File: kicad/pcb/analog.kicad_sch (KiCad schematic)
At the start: 20 parts, among them U2 74HC4051, U5 OPA354AIDBVR

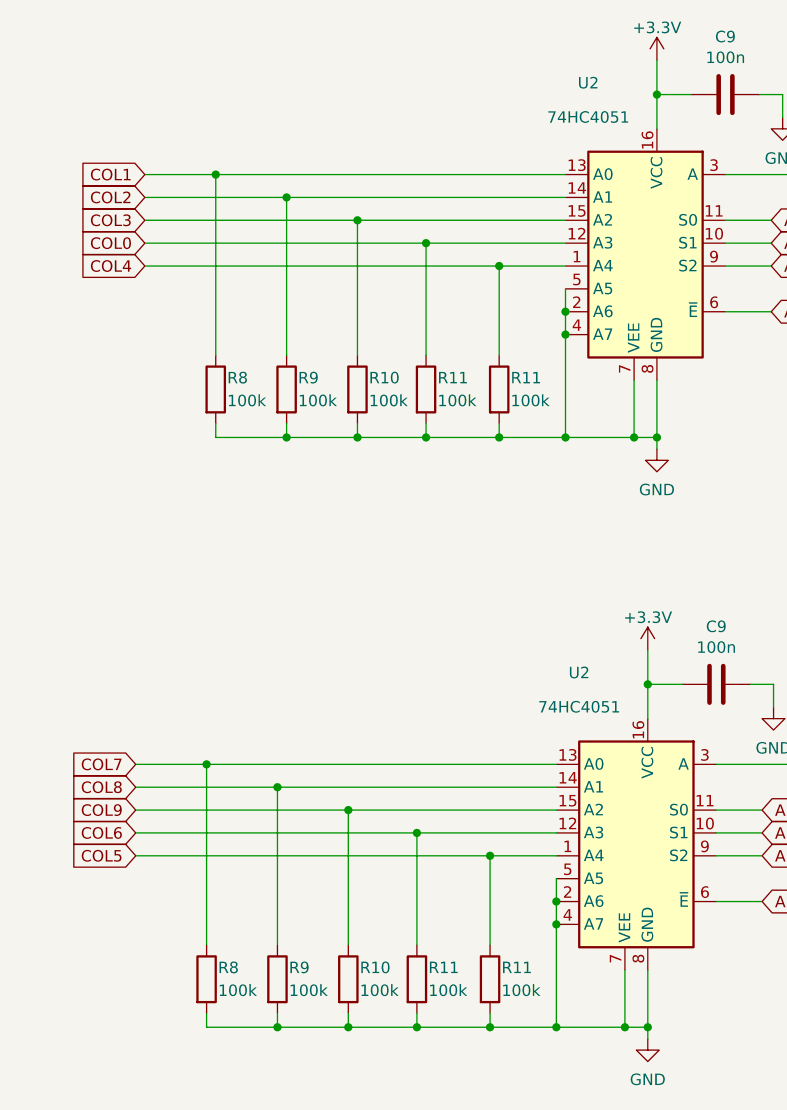
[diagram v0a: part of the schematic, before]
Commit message: rerouted pcb
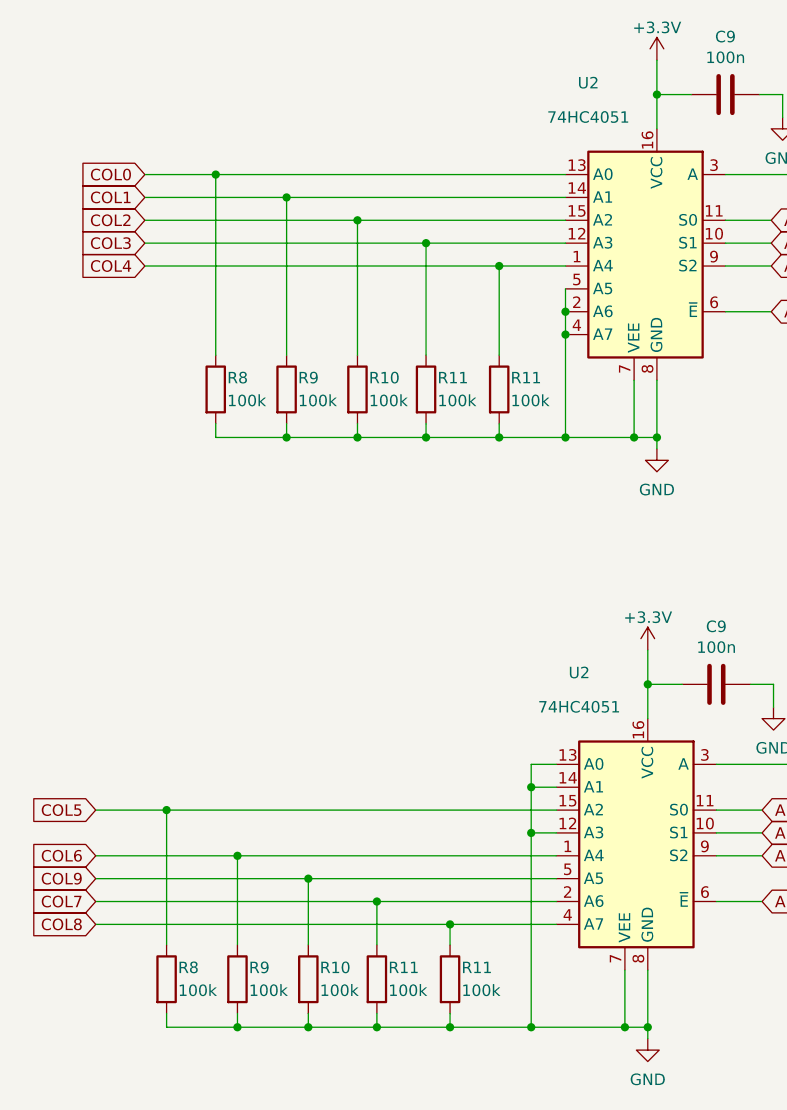
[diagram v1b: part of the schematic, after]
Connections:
- net COL0: now also R8.1, U2.13 (A0); no longer R11.1, U2.12 (A3)
- net COL1: now also R9.1, U2.14 (A1); no longer R8.1, U2.13 (A0)
- net COL2: now also R10.1, U2.15 (A2); no longer R9.1, U2.14 (A1)
- net COL3: now also R11.1, U2.12 (A3); no longer R10.1, U2.15 (A2)
- net COL5: now also R8.1, U2.15 (A2); no longer R11.1, U2.1 (A4)
- net COL6: now also R9.1, U2.1 (A4); no longer R11.1, U2.12 (A3)
- net COL7: now also R11.1, U2.2 (A6); no longer R8.1, U2.13 (A0)
- net COL8: now also R11.1, U2.4 (A7); no longer R9.1, U2.14 (A1)
- net COL9: now also U2.5 (A5); no longer U2.15 (A2)
- net GND: now also U2.12 (A3), U2.13 (A0), U2.14 (A1); no longer U2.2 (A6), U2.4 (A7), U2.5 (A5)
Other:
- moved on the sheet: R10, R11, R8, R9
